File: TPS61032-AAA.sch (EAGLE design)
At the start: 15 parts, among them IC1 TPS61032, Q1 BSS84

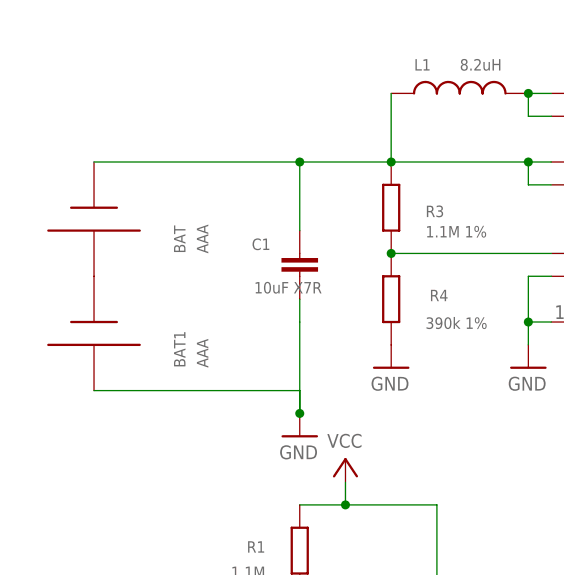
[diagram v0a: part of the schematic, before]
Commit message: Fri 17 May 2019 16:01:28 EDT - added README.md
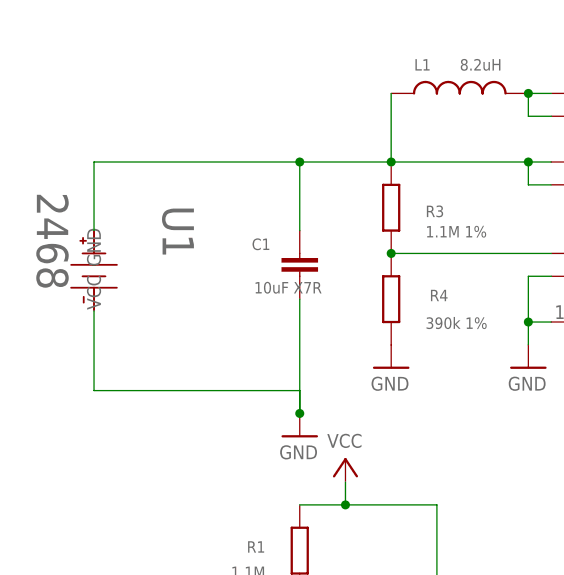
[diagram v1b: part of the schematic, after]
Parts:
- removed BAT, BAT1: AAA, adafruit:AAA
- added U1: 2468, aaa:2468
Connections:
- removed net AAA: BAT.-, BAT1.+
- net GND: now also U1.GND; no longer BAT1.-
- net VBAT: now also U1.VCC; no longer BAT.+
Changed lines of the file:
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@@
 <?xml version="1.0" encoding="utf-8"?>
 <!DOCTYPE eagle SYSTEM "eagle.dtd">
-<eagle version="9.0.0">
+<eagle version="9.0.1">
 <drawing>
 <settings>
@@
 <layer number="59" name="tCarbon" color="7" fill="1" visible="no" active="no"/>
 <layer number="60" name="bCarbon" color="7" fill="1" visible="no" active="no"/>
+<layer number="88" name="SimResults" color="9" fill="1" visible="yes" active="yes"/>
+<layer number="89" name="SimProbes" color="9" fill="1" visible="yes" active="yes"/>
 <layer number="90" name="Modules" color="7" fill="1" visible="no" active="yes"/>
 <layer number="91" name="Nets" color="2" fill="1" visible="yes" active="yes"/>
@@
 <part name="U$9" library="mw-schematic" deviceset="VCC" device=""/>
 <part name="U$10" library="mw-schematic" deviceset="VCC" device=""/>
-<part name="BAT" library="adafruit" library_urn="urn:adsk.eagle:library:420" deviceset="AAA" device="" package3d_urn="urn:adsk.eagle:package:6240648/1"/>
 <part name="C4" library="mw-passive" deviceset="C" device="0603" value="100nF"/>
-<part name="BAT1" library="adafruit" library_urn="urn:adsk.eagle:library:420" deviceset="AAA" device="" package3d_urn="urn:adsk.eagle:package:6240648/1"/>
 <part name="J1" library="SparkFun-Connectors" library_urn="urn:adsk.eagle:library:513" deviceset="CONN_02" device="PTH4" package3d_urn="urn:adsk.eagle:package:38054/1"/>
+<part name="U1" library="aaa" deviceset="2468" device=""/>
 </parts>
 <sheets>
@@
 <instance part="U$9" gate="G$1" x="119.38" y="99.06"/>
 <instance part="U$10" gate="G$1" x="30.48" y="50.8"/>
-<instance part="BAT" gate="G$1" x="2.54" y="81.28" smashed="yes" rot="R90">
-<attribute name="NAME" x="12.7" y="76.2" size="1.27" layer="95" rot="R90"/>
-<attribute name="VALUE" x="15.24" y="76.2" size="1.27" layer="96" rot="R90"/>
-</instance>
 <instance part="C4" gate="G$1" x="127" y="78.74" smashed="yes">
 <attribute name="NAME" x="123.444" y="81.661" size="1.27" layer="95"/>
 <attribute name="VALUE" x="128.524" y="81.661" size="1.27" layer="96"/>
 </instance>
-<instance part="BAT1" gate="G$1" x="2.54" y="68.58" smashed="yes" rot="R90">
-<attribute name="NAME" x="12.7" y="63.5" size="1.27" layer="95" rot="R90"/>
-<attribute name="VALUE" x="15.24" y="63.5" size="1.27" layer="96" rot="R90"/>
-</instance>
 <instance part="J1" gate="G$1" x="152.4" y="78.74" rot="R180"/>
+<instance part="U1" gate="A" x="5.08" y="81.28" rot="R270"/>
 </instances>
 <busses>
@@
 </segment>
 <segment>
-<wire x1="25.4" y1="71.12" x2="25.4" y2="68.58" width="0.1524" layer="91"/>
-<wire x1="25.4" y1="68.58" x2="25.4" y2="58.42" width="0.1524" layer="91"/>
+<wire x1="25.4" y1="71.12" x2="25.4" y2="58.42" width="0.1524" layer="91"/>
 <pinref part="C1" gate="G$1" pin="2"/>
 <pinref part="U$7" gate="G$1" pin="GND"/>
-<pinref part="BAT1" gate="G$1" pin="-"/>
 <wire x1="2.54" y1="60.96" x2="25.4" y2="60.96" width="0.1524" layer="91"/>
 <wire x1="25.4" y1="60.96" x2="25.4" y2="58.42" width="0.1524" layer="91"/>
 <junction x="25.4" y="58.42"/>
+<pinref part="U1" gate="A" pin="GND"/>
+<wire x1="2.54" y1="69.85" x2="2.54" y2="60.96" width="0.1524" layer="91"/>
 </segment>
 <segment>
@@
 <pinref part="C1" gate="G$1" pin="1"/>
 <pinref part="L1" gate="G$1" pin="1"/>
-<pinref part="BAT" gate="G$1" pin="+"/>
 <wire x1="2.54" y1="86.36" x2="25.4" y2="86.36" width="0.1524" layer="91"/>
 <junction x="25.4" y="86.36"/>
+<pinref part="U1" gate="A" pin="VCC"/>
+<wire x1="2.54" y1="78.74" x2="2.54" y2="86.36" width="0.1524" layer="91"/>
 </segment>
 </net>
@@
 </segment>
 </net>
-<net name="AAA" class="0">
-<segment>
-<pinref part="BAT" gate="G$1" pin="-"/>
-<pinref part="BAT1" gate="G$1" pin="+"/>
-</segment>
-</net>
